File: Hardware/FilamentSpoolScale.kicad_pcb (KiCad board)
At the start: 2 copper layers, 62 x 76 mm, 10 parts, among them J1 0.91 inch OLED, J2 Load Cell, J3 Screw_Terminal_01x02, SW1 SW_Push, SW2 SW_Push

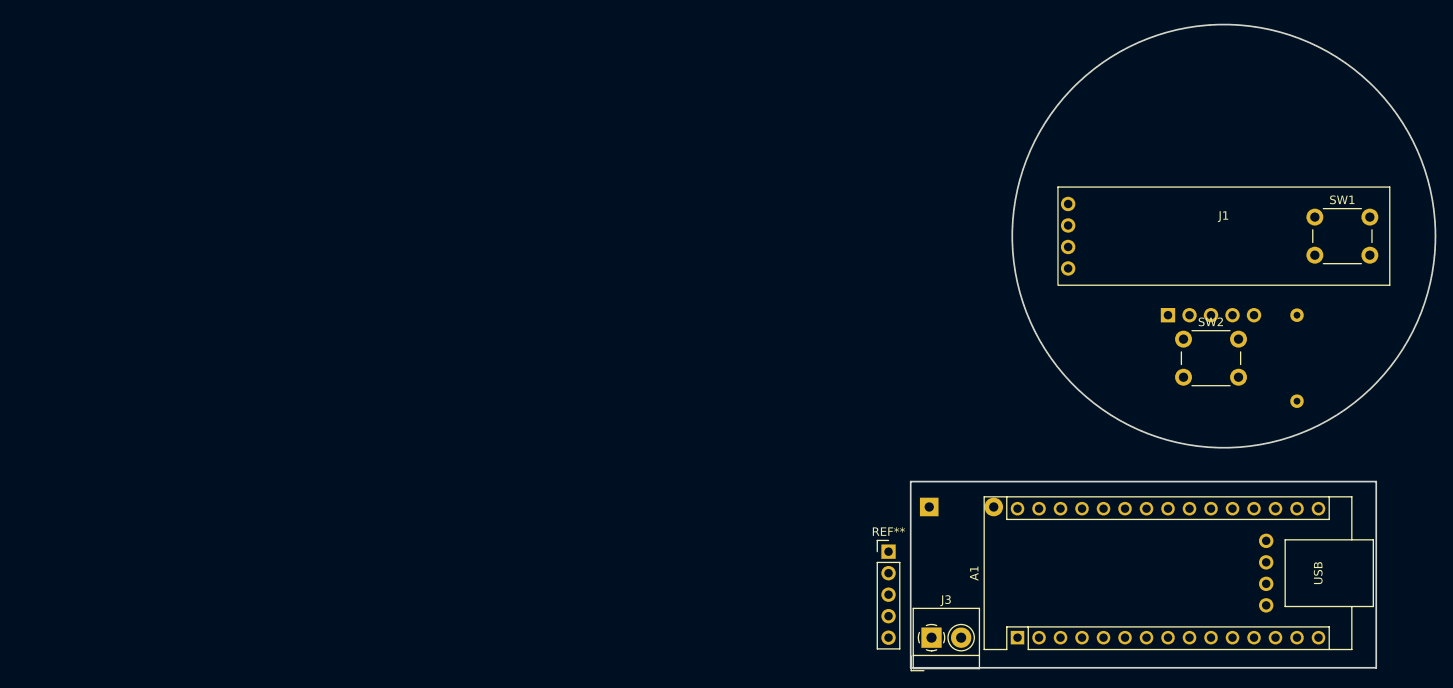
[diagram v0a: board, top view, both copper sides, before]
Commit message: Board design
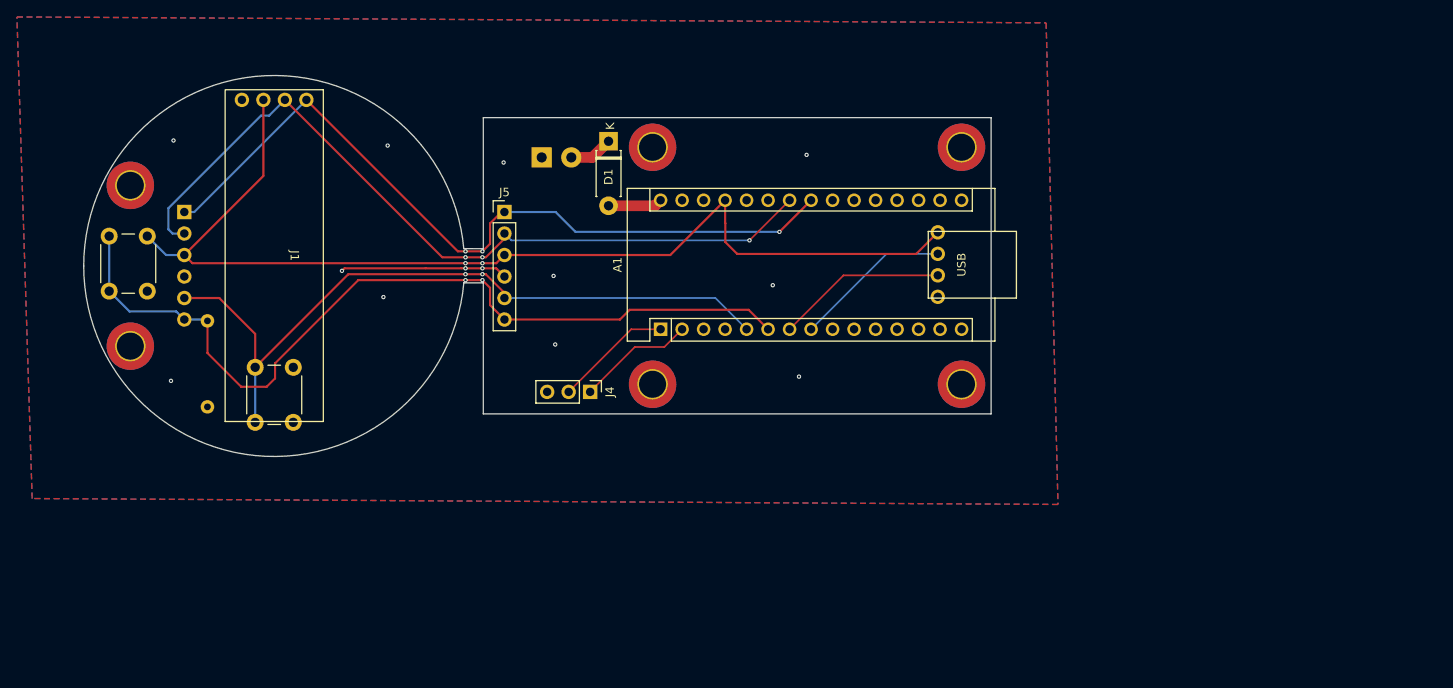
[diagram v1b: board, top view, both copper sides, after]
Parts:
- removed REF**: PinHeader_1x05_P2.54mm_Vertical, Connector_PinHeader_2.54mm:PinHeader_1x05_P2.54mm_Vertical
- removed REF**: PinHeader_1x05_P2.54mm_Horizontal, Connector_PinHeader_2.54mm:PinHeader_1x05_P2.54mm_Horizontal
- added H1: MountingHole_Pad, MountingHole:MountingHole_3.2mm_M3_DIN965_Pad_TopBottom, F.Cu at (91.5, 33.5)
- added H2: MountingHole_Pad, MountingHole:MountingHole_3.2mm_M3_DIN965_Pad_TopBottom, F.Cu at (128.0, 33.5)
- added H3: MountingHole_Pad, MountingHole:MountingHole_3.2mm_M3_DIN965_Pad_TopBottom, F.Cu at (128.0, 61.5)
- added H4: MountingHole_Pad, MountingHole:MountingHole_3.2mm_M3_DIN965_Pad_TopBottom, F.Cu at (91.5, 61.5)
- added H5: MountingHole_Pad, MountingHole:MountingHole_3.2mm_M3_DIN965_Pad_TopBottom, F.Cu at (29.8, 38.0)
- added H6: MountingHole_Pad, MountingHole:MountingHole_3.2mm_M3_DIN965_Pad_TopBottom, F.Cu at (29.8, 57.0)
- added J4: Conn_01x03, Connector_PinHeader_2.54mm:PinHeader_1x03_P2.54mm_Vertical, F.Cu at (84.1, 62.4)
- added J5: Conn_01x06, Connector_PinHeader_2.54mm:PinHeader_1x06_P2.54mm_Vertical, F.Cu at (74.0, 41.1)
- added J6: Conn_01x06, Connector_PinHeader_2.54mm:PinHeader_1x06_P2.54mm_Horizontal, B.Cu at (36.2, 41.1)
- D1: moved to F.Cu
- J3: moved to B.Cu
- R1: value R -> 10k
- moved R1 129.1 mm to (38.9, 54.0), turned to -90 degrees
- moved SW1 127.5 mm to (44.5, 66.0), turned to 90 degrees
- moved SW2 123.0 mm to (31.8, 44.0), turned to -90 degrees
- moved J1 90.8 mm to (50.6, 27.9), turned to -90 degrees
- moved J3 73.1 mm to (78.4, 34.7)
- moved D1 57.5 mm to (86.3, 32.8), turned to -90 degrees
- moved A1 55.7 mm to (92.5, 55.0)
- moved J2 53.2 mm to (125.2, 43.5)
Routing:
- net +5V: track 0.00 -> 126.6 mm, vias 0 -> 2
- net /BT2: track 0.00 -> 102.1 mm, vias 0 -> 2
- net /SCL: track 0.00 -> 94.8 mm, vias 0 -> 3
- net /SDA: track 0.00 -> 92.8 mm, vias 0 -> 3
- net /BT1: track 0.00 -> 86.2 mm, vias 0 -> 2
- net /DT: track 0.00 -> 20.1 mm
- net GND: track 0.00 -> 19.7 mm, vias 0 -> 13
- net /SCK: track 0.00 -> 18.7 mm
- net /RX: track 0.00 -> 13.9 mm
- net /TX: track 0.00 -> 13.9 mm
- net BATT: track 0.00 -> 6.42 mm
- net Net-(D1-Pad1): track 0.00 -> 5.19 mm
- added copper zone on B.Cu, net GND
- added copper zone on F.Cu, net GND
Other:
- board size 62 x 76 mm -> 107.2 x 45 mm
